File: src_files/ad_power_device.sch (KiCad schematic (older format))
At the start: 0 parts

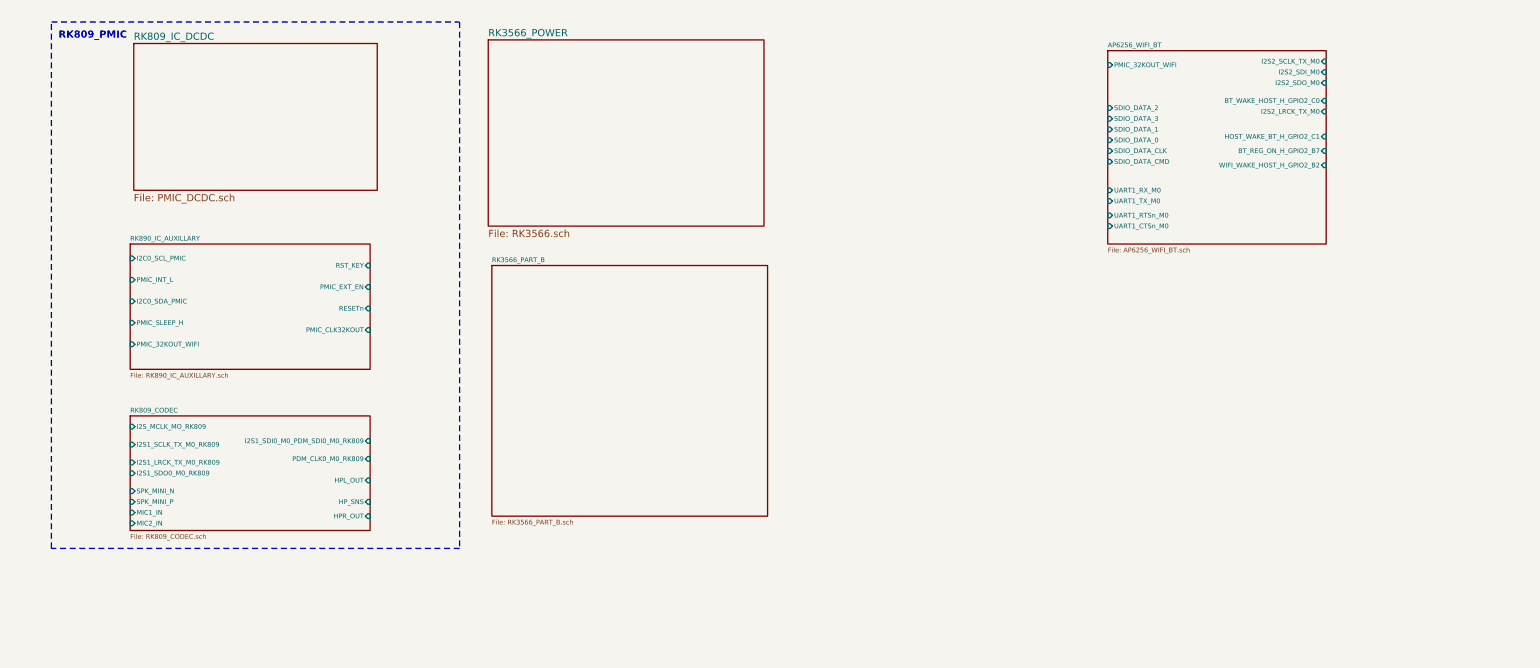
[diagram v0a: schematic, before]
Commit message: wifi module complete
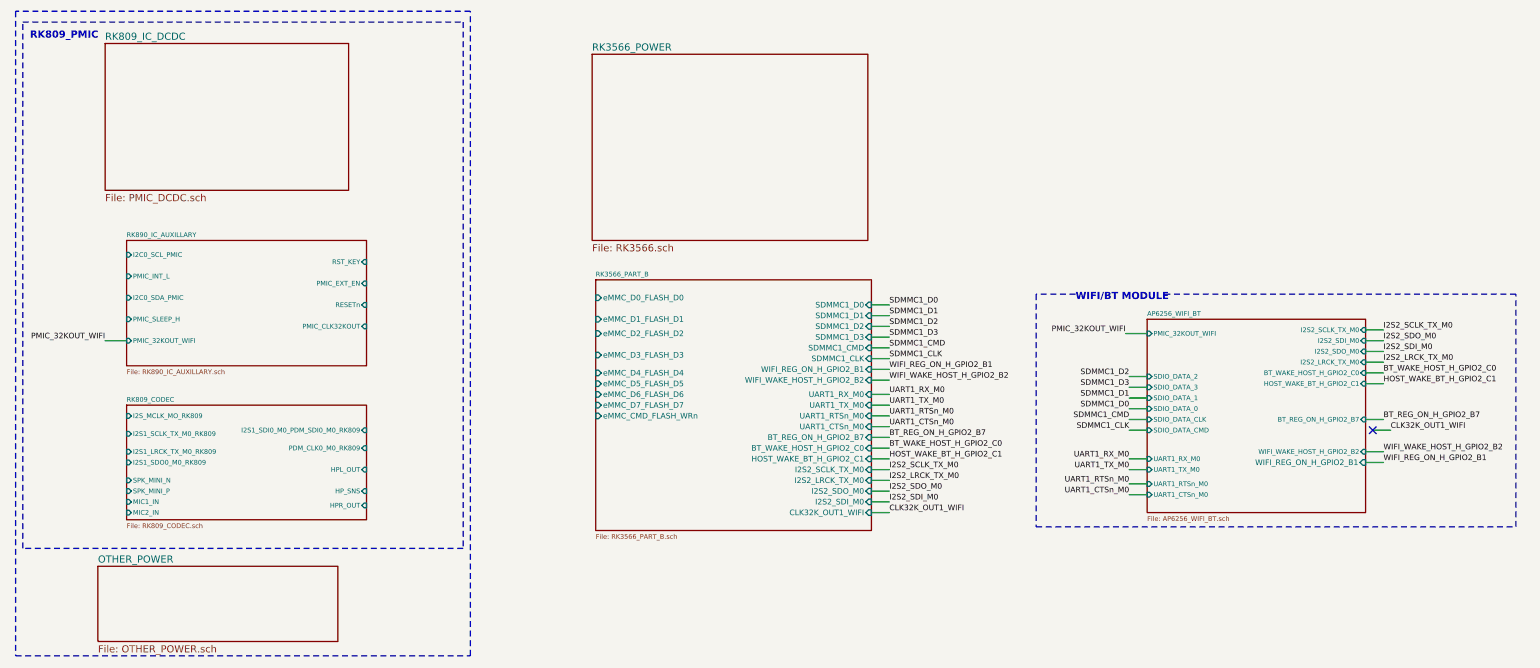
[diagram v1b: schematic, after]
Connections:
- no-connect marks 0 -> 1
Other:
- note added: "WIFI/BT MODULE"
